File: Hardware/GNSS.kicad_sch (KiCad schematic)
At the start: 20 parts, among them J1 U.FL_SMD, Q3 BSS138, U13 74HC4052D, U2 mosaic-X5

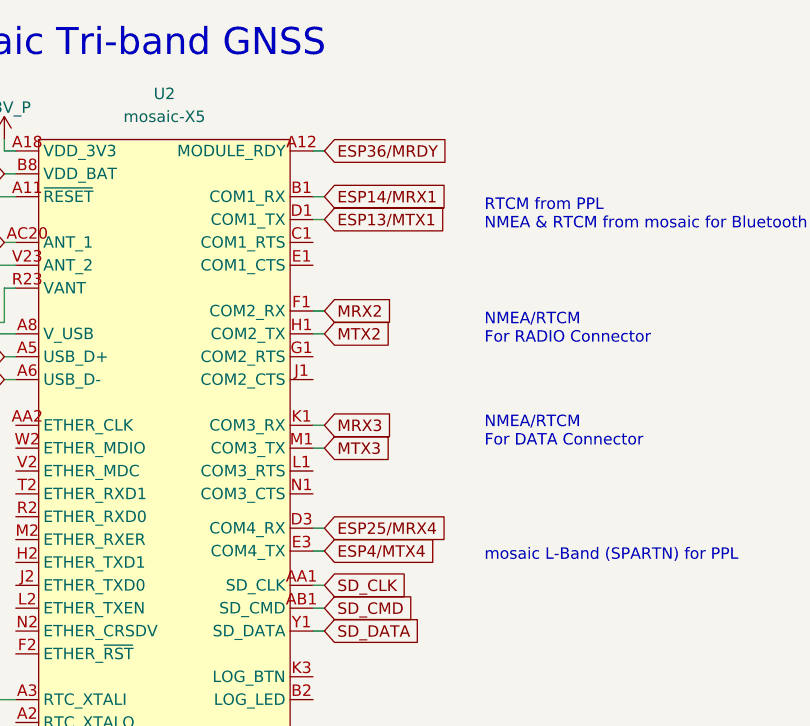
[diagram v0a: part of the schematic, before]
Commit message: Work in progress...
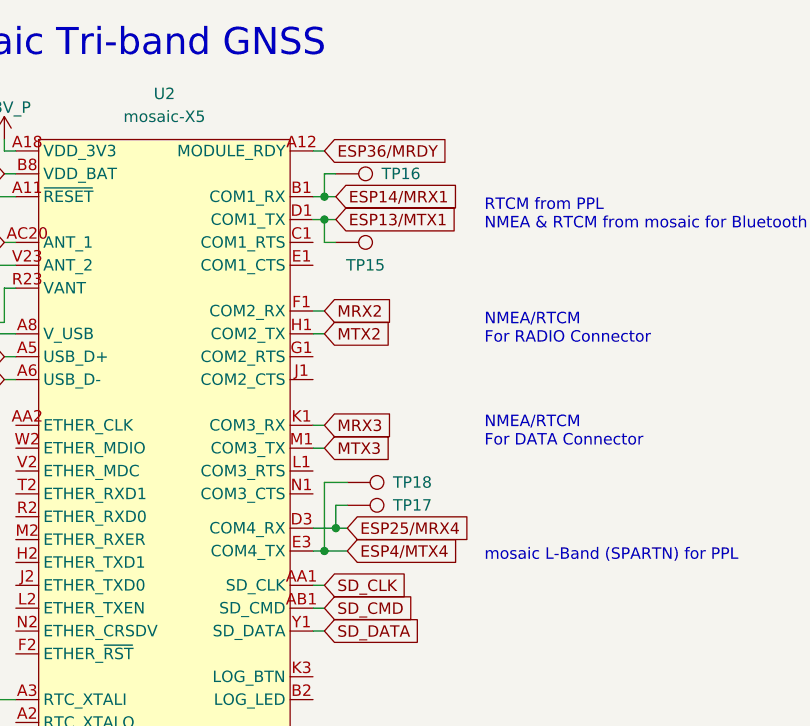
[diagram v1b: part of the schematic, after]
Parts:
- added TP15, TP16, TP17, TP18: 1.0mm, SparkFun-Connector:TestPoint-1.0mm, symbol SparkFun-Connector:TestPoint_1.0mm
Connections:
- net ESP13/MTX1: now also TP15.1
- net ESP14/MRX1: now also TP16.1
- net ESP25/MRX4: now also TP17.1
- net ESP4/MTX4: now also TP18.1
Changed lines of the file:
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@@
   (junction (at 57.15 97.79) (diameter 0) (color 0 0 0 0)
   )
+  (junction (at 92.71 36.83) (diameter 0) (color 0 0 0 0)
+  )
   (junction (at 231.14 128.27) (diameter 0) (color 0 0 0 0)
   )
+  (junction (at 92.71 34.29) (diameter 0) (color 0 0 0 0)
+  )
   (junction (at 210.82 128.27) (diameter 0) (color 0 0 0 0)
   )
@@
   (junction (at 48.26 113.03) (diameter 0) (color 0 0 0 0)
   )
+  (junction (at 93.98 71.12) (diameter 0) (color 0 0 0 0)
+  )
   (junction (at 36.83 34.29) (diameter 0) (color 0 0 0 0)
   )
+  (junction (at 92.71 73.66) (diameter 0) (color 0 0 0 0)
+  )
   (wire (pts (xy 91.44 77.47) (xy 92.71 77.47))
     (stroke (width 0) (type default))
@@
     (stroke (width 0) (type default))
   )
+  (wire (pts (xy 95.25 66.04) (xy 92.71 66.04))
+    (stroke (width 0) (type default))
+  )
   (wire (pts (xy 22.86 86.36) (xy 22.86 85.09))
     (stroke (width 0) (type default))
@@
     (stroke (width 0) (type default))
   )
+  (wire (pts (xy 92.71 66.04) (xy 92.71 73.66))
+    (stroke (width 0) (type default))
+  )
   (wire (pts (xy 57.15 97.79) (xy 58.42 97.79))
     (stroke (width 0) (type default))
   )
+  (wire (pts (xy 92.71 31.75) (xy 92.71 34.29))
+    (stroke (width 0) (type default))
+  )
   (wire (pts (xy 55.88 97.79) (xy 57.15 97.79))
     (stroke (width 0) (type default))
   )
+  (wire (pts (xy 93.98 71.12) (xy 95.25 71.12))
+    (stroke (width 0) (type default))
+  )
   (wire (pts (xy 210.82 128.27) (xy 212.09 128.27))
     (stroke (width 0) (type default))
@@
     (stroke (width 0) (type default))
   )
-  (wire (pts (xy 91.44 71.12) (xy 92.71 71.12))
+  (wire (pts (xy 91.44 71.12) (xy 93.98 71.12))
     (stroke (width 0) (type default))
   )
@@
     (stroke (width 0) (type default))
   )
+  (wire (pts (xy 92.71 34.29) (xy 93.98 34.29))
+    (stroke (width 0) (type default))
+  )
   (wire (pts (xy 29.21 71.12) (xy 29.21 69.85))
     (stroke (width 0) (type default))
@@
     (stroke (width 0) (type default))
   )
+  (wire (pts (xy 92.71 36.83) (xy 92.71 39.37))
+    (stroke (width 0) (type default))
+  )
   (wire (pts (xy 223.52 128.27) (xy 231.14 128.27))
     (stroke (width 0) (type default))
@@
     (stroke (width 0) (type default))
   )
+  (wire (pts (xy 93.98 39.37) (xy 92.71 39.37))
+    (stroke (width 0) (type default))
+  )
   (wire (pts (xy 210.82 38.1) (xy 214.63 38.1))
     (stroke (width 0) (type default))
   )
+  (wire (pts (xy 93.98 68.58) (xy 93.98 71.12))
+    (stroke (width 0) (type default))
+  )
   (wire (pts (xy 34.29 34.29) (xy 36.83 34.29))
     (stroke (width 0) (type default))
@@
     (stroke (width 0) (type default))
   )
+  (wire (pts (xy 92.71 73.66) (xy 95.25 73.66))
+    (stroke (width 0) (type default))
+  )
   (wire (pts (xy 36.83 24.13) (xy 36.83 25.4))
     (stroke (width 0) (type default))
@@
     (stroke (width 0) (type default))
   )
+  (wire (pts (xy 95.25 68.58) (xy 93.98 68.58))
+    (stroke (width 0) (type default))
+  )
   (wire (pts (xy 87.63 167.64) (xy 86.36 167.64))
     (stroke (width 0) (type default))
@@
     (stroke (width 0) (type default))
   )
+  (wire (pts (xy 92.71 36.83) (xy 93.98 36.83))
+    (stroke (width 0) (type default))
+  )
   (wire (pts (xy 91.44 80.01) (xy 92.71 80.01))
     (stroke (width 0) (type default))
@@
   )
   (wire (pts (xy 57.15 44.45) (xy 57.15 48.26))
+    (stroke (width 0) (type default))
+  )
+  (wire (pts (xy 93.98 31.75) (xy 92.71 31.75))
     (stroke (width 0) (type default))
   )
@@
     )
   )
-  (global_label "ESP14{slash}MRX1" (shape input) (at 92.71 34.29 0) (fields_autoplaced)
-    (effects (font (size 1.27 1.27)) (justify left))
-    (property "Intersheetrefs" "${INTERSHEET_REFS}" (at 107.0041 34.29 0)
+  (global_label "ESP14{slash}MRX1" (shape input) (at 93.98 34.29 0) (fields_autoplaced)
+    (effects (font (size 1.27 1.27)) (justify left))
+    (property "Intersheetrefs" "${INTERSHEET_REFS}" (at 108.2741 34.29 0)
       (effects (font (size 1.27 1.27)) (justify left) hide)
     )
@@
     )
   )
-  (global_label "ESP25{slash}MRX4" (shape input) (at 92.71 71.12 0) (fields_autoplaced)
-    (effects (font (size 1.27 1.27)) (justify left))
-    (property "Intersheetrefs" "${INTERSHEET_REFS}" (at 108.2136 71.12 0)
+  (global_label "ESP25{slash}MRX4" (shape input) (at 95.25 71.12 0) (fields_autoplaced)
+    (effects (font (size 1.27 1.27)) (justify left))
+    (property "Intersheetrefs" "${INTERSHEET_REFS}" (at 110.7536 71.12 0)
       (effects (font (size 1.27 1.27)) (justify left) hide)
     )
@@
     )
   )
-  (global_label "ESP4{slash}MTX4" (shape input) (at 92.71 73.66 0) (fields_autoplaced)
-    (effects (font (size 1.27 1.27)) (justify left))
-    (property "Intersheetrefs" "${INTERSHEET_REFS}" (at 106.7017 73.66 0)
+  (global_label "ESP4{slash}MTX4" (shape input) (at 95.25 73.66 0) (fields_autoplaced)
+    (effects (font (size 1.27 1.27)) (justify left))
+    (property "Intersheetrefs" "${INTERSHEET_REFS}" (at 109.2417 73.66 0)
       (effects (font (size 1.27 1.27)) (justify left) hide)
     )
@@
     )
   )
-  (global_label "ESP13{slash}MTX1" (shape input) (at 92.71 36.83 0) (fields_autoplaced)
-    (effects (font (size 1.27 1.27)) (justify left))
-    (property "Intersheetrefs" "${INTERSHEET_REFS}" (at 106.7017 36.83 0)
+  (global_label "ESP13{slash}MTX1" (shape input) (at 93.98 36.83 0) (fields_autoplaced)
+    (effects (font (size 1.27 1.27)) (justify left))
+    (property "Intersheetrefs" "${INTERSHEET_REFS}" (at 107.9717 36.83 0)
       (effects (font (size 1.27 1.27)) (justify left) hide)
     )
@@
     )
   )
+  (symbol (lib_id "SparkFun-Connector:TestPoint_1.0mm") (at 93.98 31.75 270) (unit 1)
+    (in_bom yes) (on_board yes) (dnp no) (fields_autoplaced)
+    (property "Reference" "TP16" (at 99.06 31.75 90)
+      (effects (font (size 1.27 1.27)) (justify left))
+    )
+    (property "Value" "1.0mm" (at 90.17 31.75 0)
+      (effects (font (size 1.27 1.27)) hide)
+    )
+    (property "Footprint" "SparkFun-Connector:TestPoint-1.0mm" (at 87.63 31.75 0)
+      (effects (font (size 1.27 1.27)) hide)
+    )
+    (property "Datasheet" "~" (at 86.36 31.75 0)
+      (effects (font (size 1.27 1.27)) hide)
+    )
+    (pin "1")
+    (instances
+      (project "SparkFun_RTK_Facet_mosaic"
+        (path "/e3dd3ae4-244d-4cba-9cca-5d2abf83f29a/1004b21d-c362-4c5d-adad-4952c3ff3811"
+          (reference "TP16") (unit 1)
+        )
+      )
+    )
+  )
   (symbol (lib_id "SparkFun-Resistor:10k_0402") (at 53.34 115.57 0) (unit 1)
     (in_bom yes) (on_board yes) (dnp no)
@@
         (path "/e3dd3ae4-244d-4cba-9cca-5d2abf83f29a/1004b21d-c362-4c5d-adad-4952c3ff3811"
           (reference "#PWR010") (unit 1)
+        )
+      )
+    )
+  )
+  (symbol (lib_id "SparkFun-Connector:TestPoint_1.0mm") (at 93.98 39.37 270) (unit 1)
+    (in_bom yes) (on_board yes) (dnp no) (fields_autoplaced)
+    (property "Reference" "TP15" (at 97.282 41.91 90)
+      (effects (font (size 1.27 1.27)))
+    )
+    (property "Value" "1.0mm" (at 90.17 39.37 0)
+      (effects (font (size 1.27 1.27)) hide)
+    )
+    (property "Footprint" "SparkFun-Connector:TestPoint-1.0mm" (at 87.63 39.37 0)
+      (effects (font (size 1.27 1.27)) hide)
+    )
+    (property "Datasheet" "~" (at 86.36 39.37 0)
+      (effects (font (size 1.27 1.27)) hide)
+    )
+    (pin "1")
+    (instances
+      (project "SparkFun_RTK_Facet_mosaic"
+        (path "/e3dd3ae4-244d-4cba-9cca-5d2abf83f29a/1004b21d-c362-4c5d-adad-4952c3ff3811"
+          (reference "TP15") (unit 1)
         )
       )
@@
     )
   )
+  (symbol (lib_id "SparkFun-Connector:TestPoint_1.0mm") (at 95.25 68.58 270) (unit 1)
+    (in_bom yes) (on_board yes) (dnp no) (fields_autoplaced)
+    (property "Reference" "TP17" (at 100.33 68.58 90)
+      (effects (font (size 1.27 1.27)) (justify left))
+    )
+    (property "Value" "1.0mm" (at 91.44 68.58 0)
+      (effects (font (size 1.27 1.27)) hide)
+    )
+    (property "Footprint" "SparkFun-Connector:TestPoint-1.0mm" (at 88.9 68.58 0)
+      (effects (font (size 1.27 1.27)) hide)
+    )
+    (property "Datasheet" "~" (at 87.63 68.58 0)
+      (effects (font (size 1.27 1.27)) hide)
+    )
+    (pin "1")
+    (instances
+      (project "SparkFun_RTK_Facet_mosaic"
+        (path "/e3dd3ae4-244d-4cba-9cca-5d2abf83f29a/1004b21d-c362-4c5d-adad-4952c3ff3811"
+          (reference "TP17") (unit 1)
+        )
+      )
+    )
+  )
   (symbol (lib_id "SparkFun-Capacitor:22uF_0603_6.3V_20%") (at 29.21 66.04 0) (unit 1)
     (in_bom yes) (on_board yes) (dnp no) (fields_autoplaced)
@@
         )
       )
+    )
+  )
+  (symbol (lib_id "SparkFun-Connector:TestPoint_1.0mm") (at 95.25 66.04 270) (unit 1)
+    (in_bom yes) (on_board yes) (dnp no) (fields_autoplaced)
+    (property "Reference" "TP18" (at 100.33 66.04 90)
+      (effects (font (size 1.27 1.27)) (justify left))
+    )
+    (property "Value" "1.0mm" (at 91.44 66.04 0)
+      (effects (font (size 1.27 1.27)) hide)
+    )
+    (property "Footprint" "SparkFun-Connector:TestPoint-1.0mm" (at 88.9 66.04 0)
+      (effects (font (size 1.27 1.27)) hide)
+    )
+    (property "Datasheet" "~" (at 87.63 66.04 0)
+      (effects (font (size 1.27 1.27)) hide)
+    )
+    (pin "1")
+    (instances
+      (project "SparkFun_RTK_Facet_mosaic"
+        (path "/e3dd3ae4-244d-4cba-9cca-5d2abf83f29a/1004b21d-c362-4c5d-adad-4952c3ff3811"
+          (reference "TP18") (unit 1)
+        )
+      )
